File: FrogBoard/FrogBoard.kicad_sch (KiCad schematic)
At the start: 61 parts, among them J1 Conn_01x10, J10 Conn_01x01, J11 Conn_01x01, J12 Conn_01x02, J13 Conn_01x01, J14 Conn_01x01, J15 Conn_01x01, J16 Conn_01x01, J17 Conn_01x01, J18 Conn_01x01, J19 Conn_01x01, J2 Conn_01x04, J20 Conn_01x01, J21 Conn_01x01, J22 Conn_01x01, J23 Conn_01x01, J24 Conn_01x01, J25 Conn_01x01, J27 Conn_01x01, J28 Conn_01x01, J3 USB_C_Receptacle_USB2.0_16P, J30 Conn_01x02, J4 Stickbox, J5 Conn_01x03_Socket, J6 Conn_01x02, J7 Conn_01x02, J8 Conn_01x01, J9 Conn_01x01, U1 STM32L432KBUx, U2 USBLC6-2P6, U3 MCP1700T-3302E, U4 BL1555

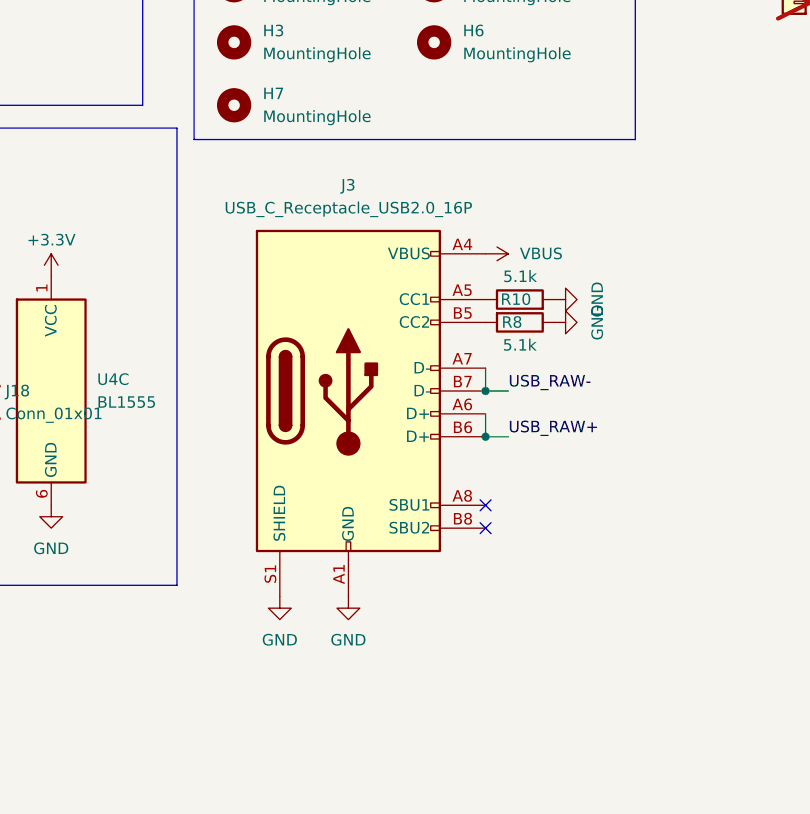
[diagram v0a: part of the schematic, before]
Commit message: Update footprint and put back micro USB
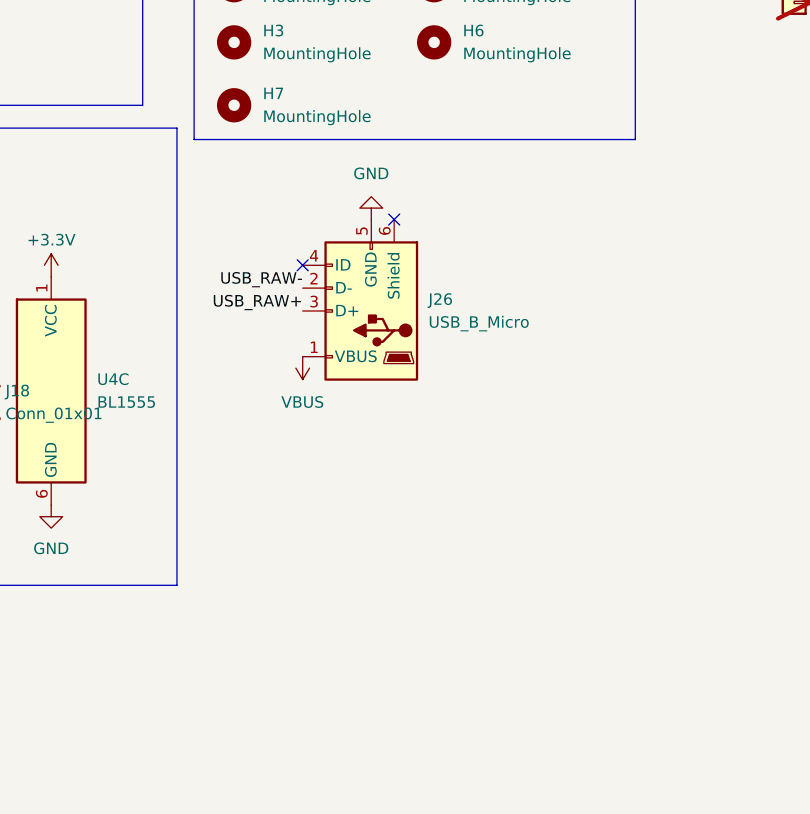
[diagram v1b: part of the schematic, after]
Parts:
- removed J3: USB_C_Receptacle_USB2.0_16P, FrogBoard_footprints:CONN16_C16PIN_SHN, symbol Connector:USB_C_Receptacle_USB2.0_16P
- removed R10, R8: 5.1k, Resistor_SMD:R_0603_1608Metric_Pad0.98x0.95mm_HandSolder, symbol Device:R
- added J26: USB_B_Micro, FrogBoard_footprints:AMPHENOL_10118194-0001LF, symbol Connector:USB_B_Micro
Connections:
- net GND: now also J26.5 (GND)
- net USB_RAW+: now also J26.3 (D+)
- net USB_RAW-: now also J26.2 (D-)
- net VBUS: now also J26.1 (VBUS)

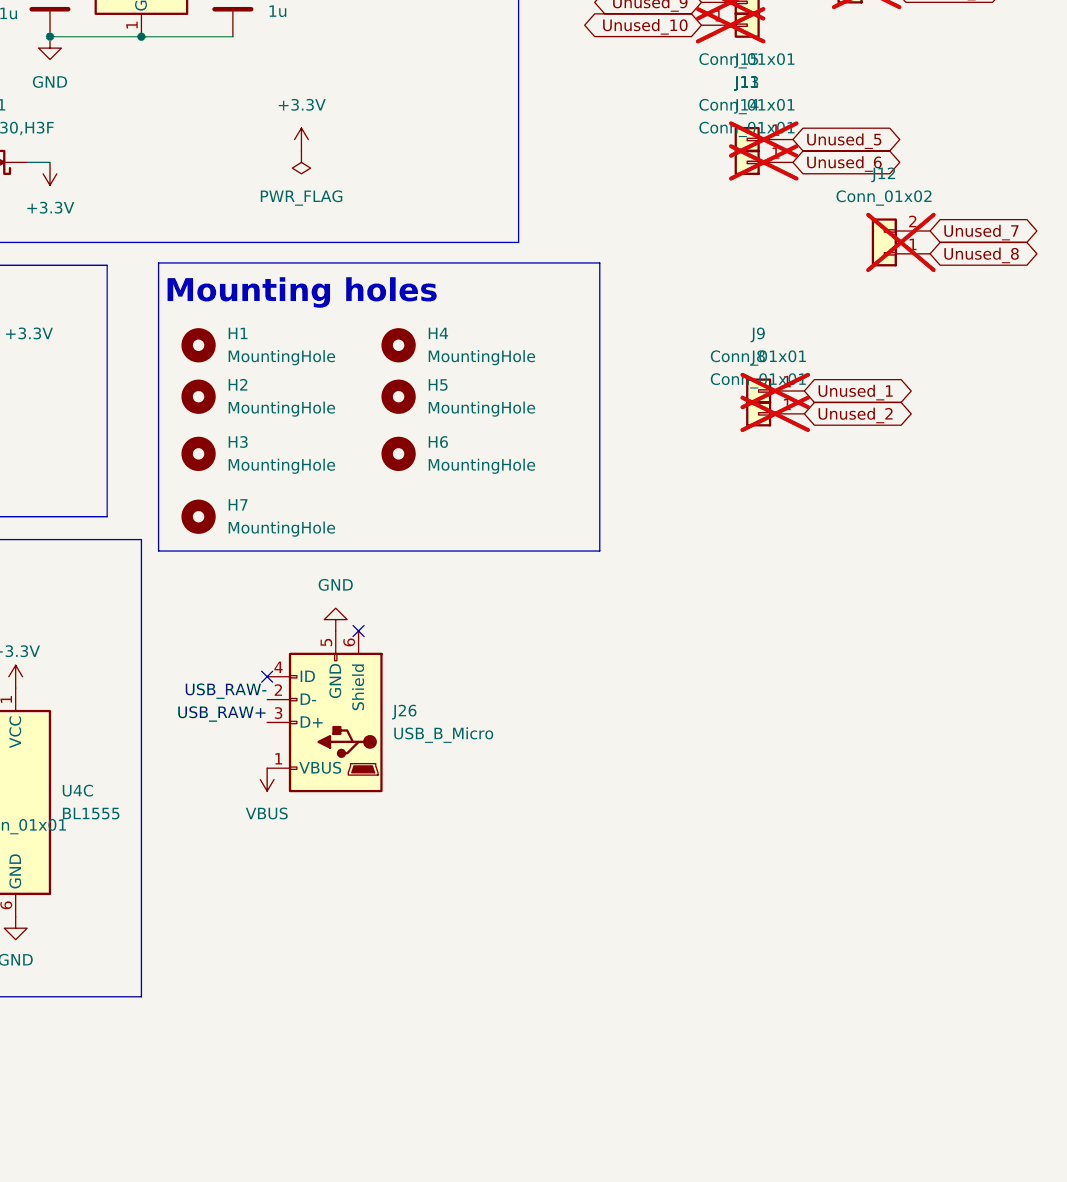
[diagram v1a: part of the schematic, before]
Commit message: bulk rounting done
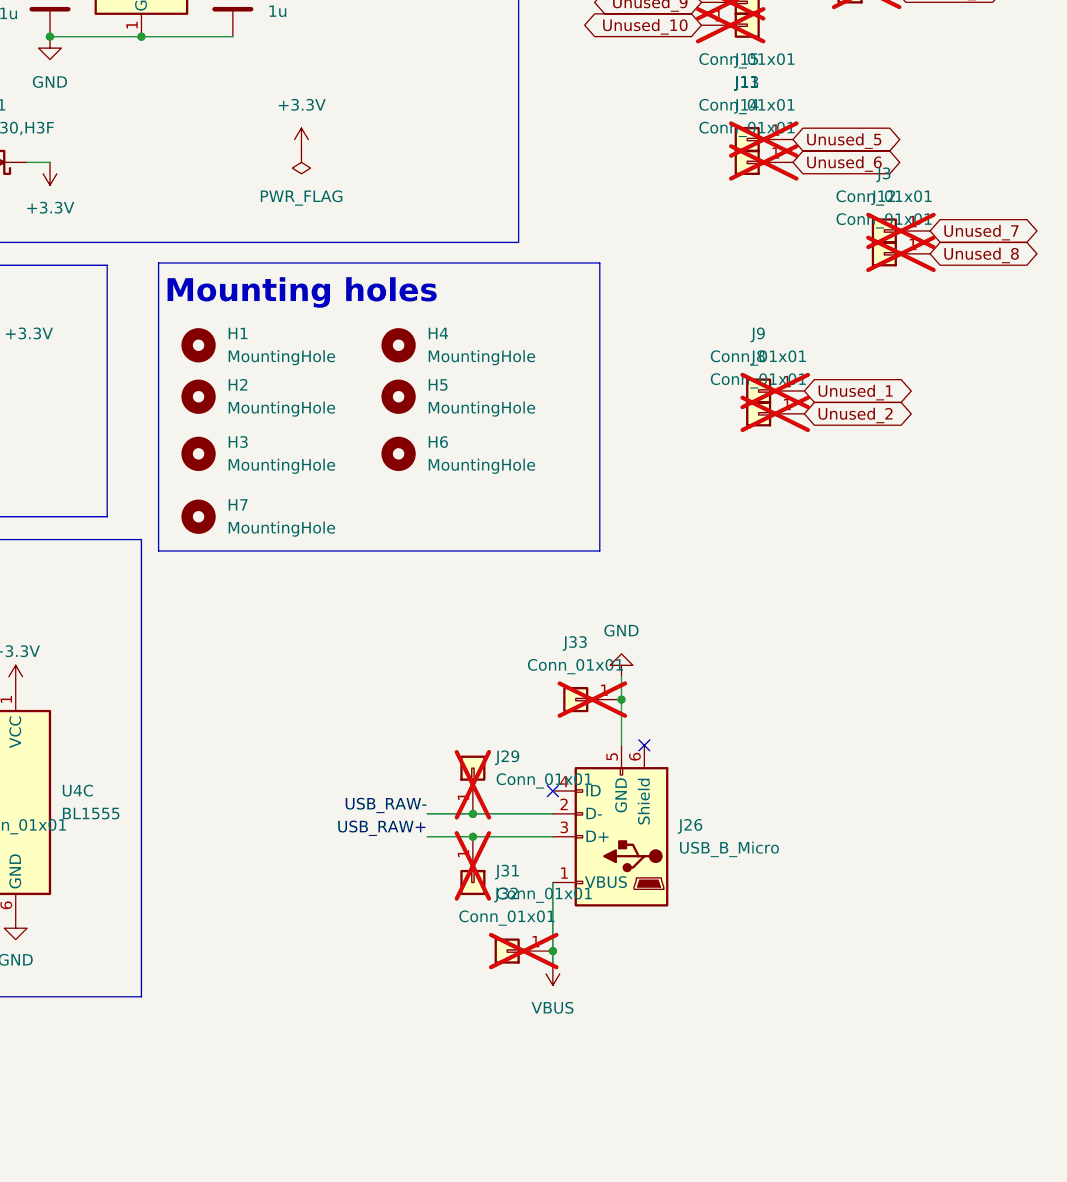
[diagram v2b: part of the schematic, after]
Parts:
- removed J12: Conn_01x02, FrogBoard_footprints:PinHeader_1x02_P1.00mm_Vertical_Neutral_No_Coutryard, symbol Connector_Generic:Conn_01x02
- added J12, J29, J3, J31, J32, J33: Conn_01x01, FrogBoard_footprints:FrogBoard_PinHeader_1x01_P1.00mm_Vertical, symbol Connector_Generic:Conn_01x01
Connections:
- net GND: now also J33.1 (Pin_1)
- net USB_RAW+: now also J31.1 (Pin_1)
- net USB_RAW-: now also J29.1 (Pin_1)
- net Unused_7: now also J3.1 (Pin_1)
- net Unused_8: now also J12.1 (Pin_1)
- net VBUS: now also J32.1 (Pin_1)
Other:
- moved on the sheet: J26
